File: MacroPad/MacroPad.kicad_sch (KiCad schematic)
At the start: 30 parts, among them J101 USB_B_Micro, J102 ICSP, SW101 SW_Push, SW102 SW_Push, SW103 SW_Push, SW104 SW_Push, SW105 SW_Push, SW106 SW_Push, U101 ATmega32U4-A, Y101 16MHz

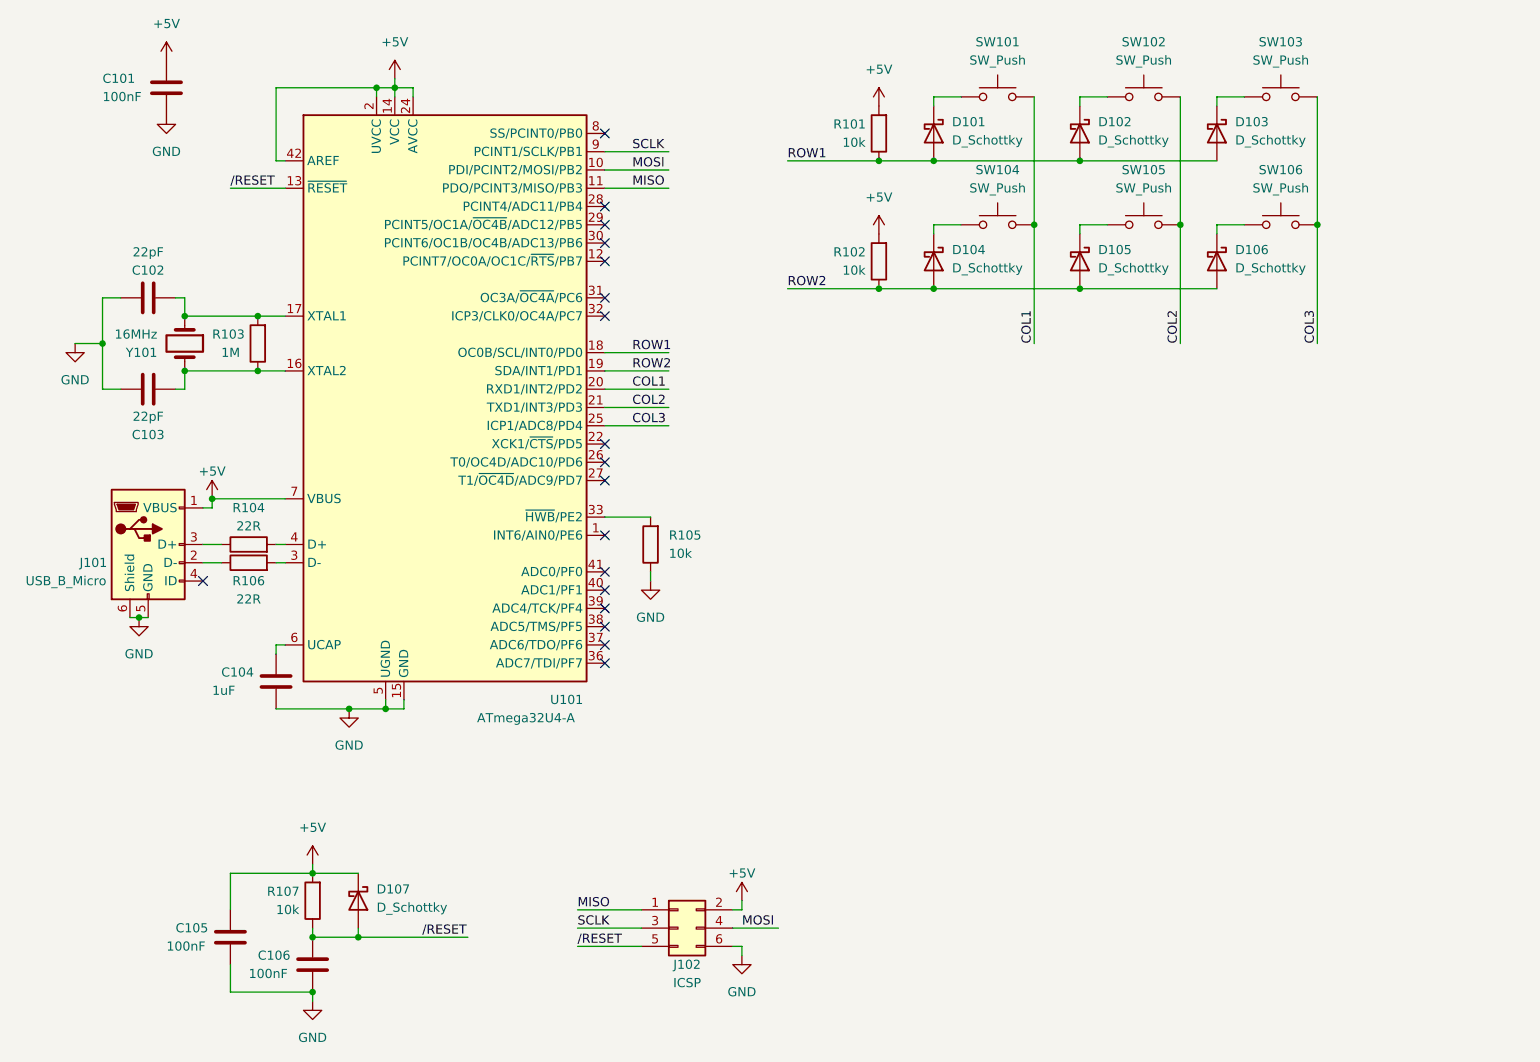
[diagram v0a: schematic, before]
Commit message: Fixed microcontroller hooks
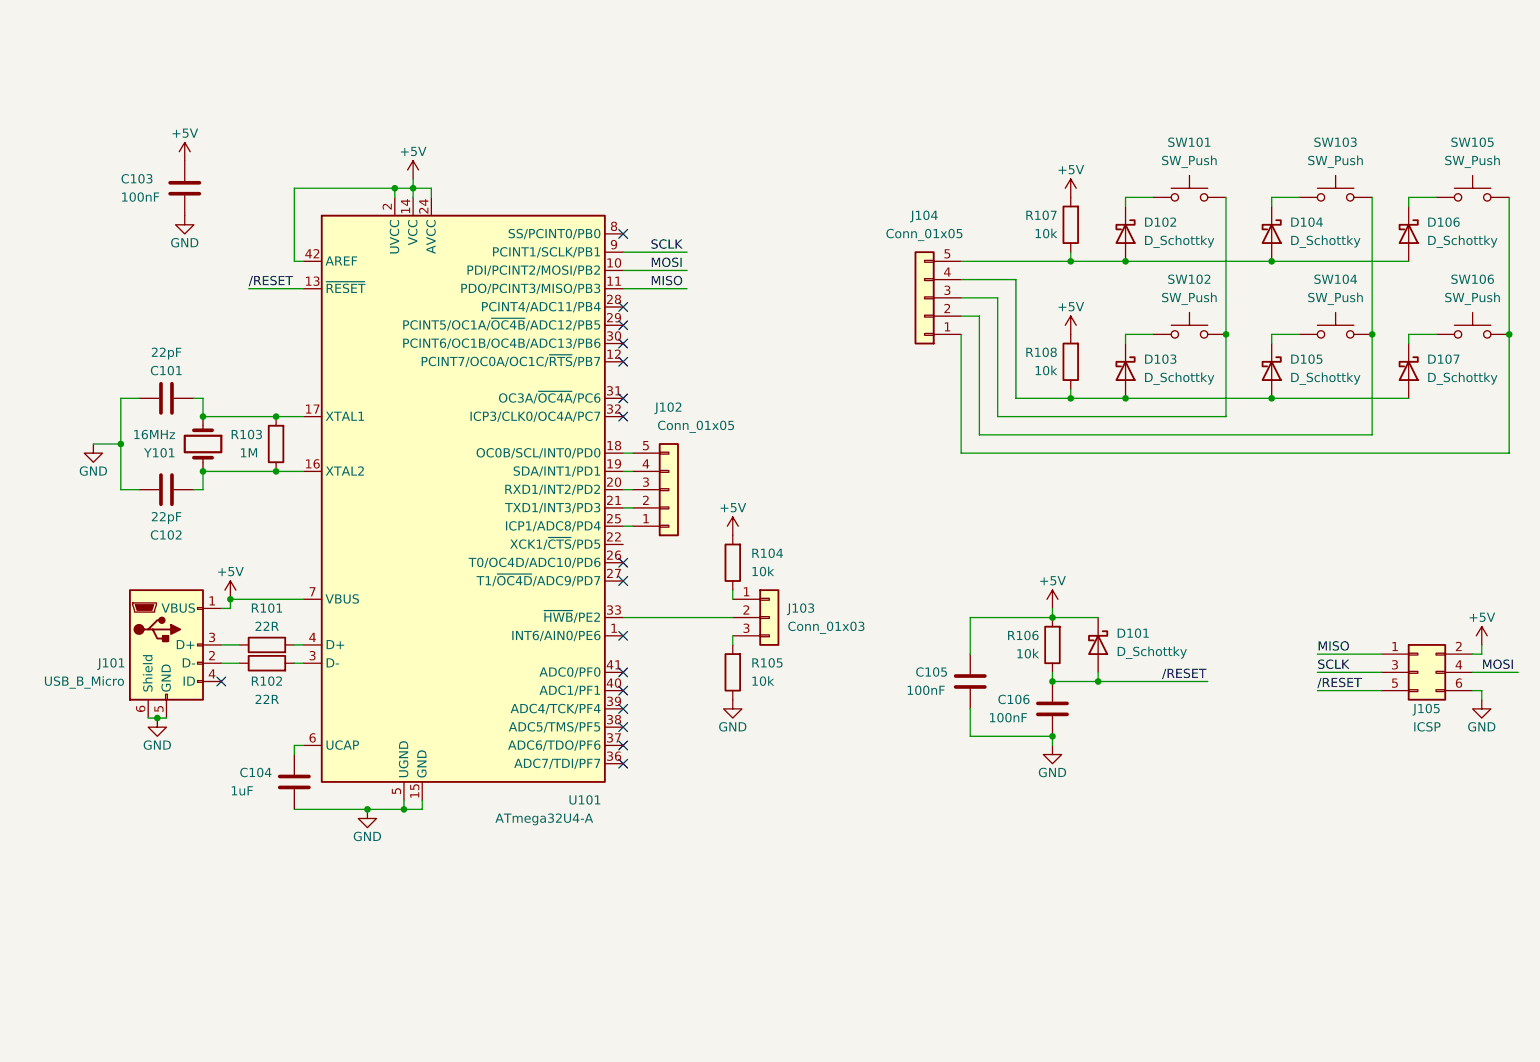
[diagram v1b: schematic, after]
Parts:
- added J102, J104: Conn_01x05, Connector_PinHeader_2.54mm:PinHeader_1x05_P2.54mm_Vertical, symbol Connector_Generic:Conn_01x05
- added J103: Conn_01x03, symbol Connector_Generic:Conn_01x03
- added R104: 10k, Resistor_THT:R_Axial_DIN0207_L6.3mm_D2.5mm_P7.62mm_Horizontal, symbol Device:R
- renumbered C102 to C101, C103 to C102, C101 to C103, D107 to D101, D101 to D102, D104 to D103, D102 to D104, D103 to D106, D106 to D107, J102 to J105, R104 to R101, R106 to R102, R107 to R106, R101 to R107, R102 to R108, SW104 to SW102, SW102 to SW103, SW105 to SW104, SW103 to SW105
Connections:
- net +5V: now also R104.2
- net at U101.33 (~{HWB}/PE2): now also J103.2 (Pin_2); no longer R105.2
- net COL1: no longer names the net of SW101.2, SW102.2
- net COL1: now also J104.3 (Pin_3); no longer U101.20 (RXD1/INT2/PD2)
- net COL2: no longer names the net of SW103.2, SW104.2
- net COL2: now also J104.2 (Pin_2); no longer U101.21 (TXD1/INT3/PD3)
- net COL3: no longer names the net of SW105.2, SW106.2
- net COL3: now also J104.1 (Pin_1); no longer U101.25 (ICP1/ADC8/PD4)
- net ROW1: no longer names the net of D102.2 (A), D104.2 (A), D106.2 (A), R107.1
- net ROW1: now also J104.5 (Pin_5); no longer U101.18 (OC0B/SCL/INT0/PD0)
- net ROW2: no longer names the net of D103.2 (A), D105.2 (A), D107.2 (A), R108.1
- net ROW2: now also J104.4 (Pin_4); no longer U101.19 (SDA/INT1/PD1)
- new net: J103.1 (Pin_1), R104.1
- new net: J103.3 (Pin_3), R105.2
- new net: J102.5 (Pin_5), U101.18 (OC0B/SCL/INT0/PD0)
- new net: J102.4 (Pin_4), U101.19 (SDA/INT1/PD1)
- new net: J102.3 (Pin_3), U101.20 (RXD1/INT2/PD2)
- new net: J102.2 (Pin_2), U101.21 (TXD1/INT3/PD3)
- new net: J102.1 (Pin_1), U101.25 (ICP1/ADC8/PD4)
- no-connect marks 18 -> 17
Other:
- moved on the sheet: C101, C102, C103, C104, C105, C106, D101, D102, D103, D104, D105, D106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
